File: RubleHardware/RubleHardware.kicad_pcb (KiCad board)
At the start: 4 copper layers, 62 x 46 mm, 49 parts, among them IC1 LTC3780EUH#PBF, J1_IN1 Conn_01x08_Male, J2_OUT1 Conn_01x08_Male

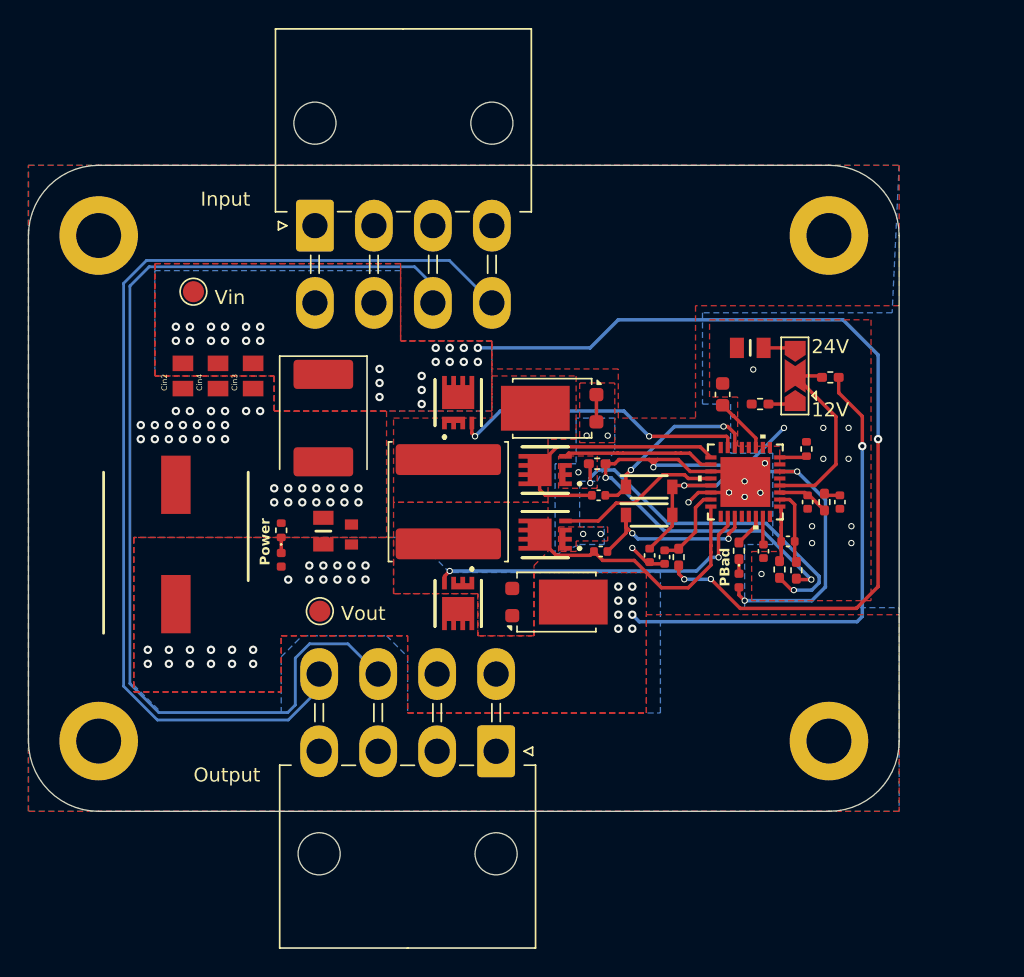
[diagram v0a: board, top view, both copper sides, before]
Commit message: feat: v0.4 ready
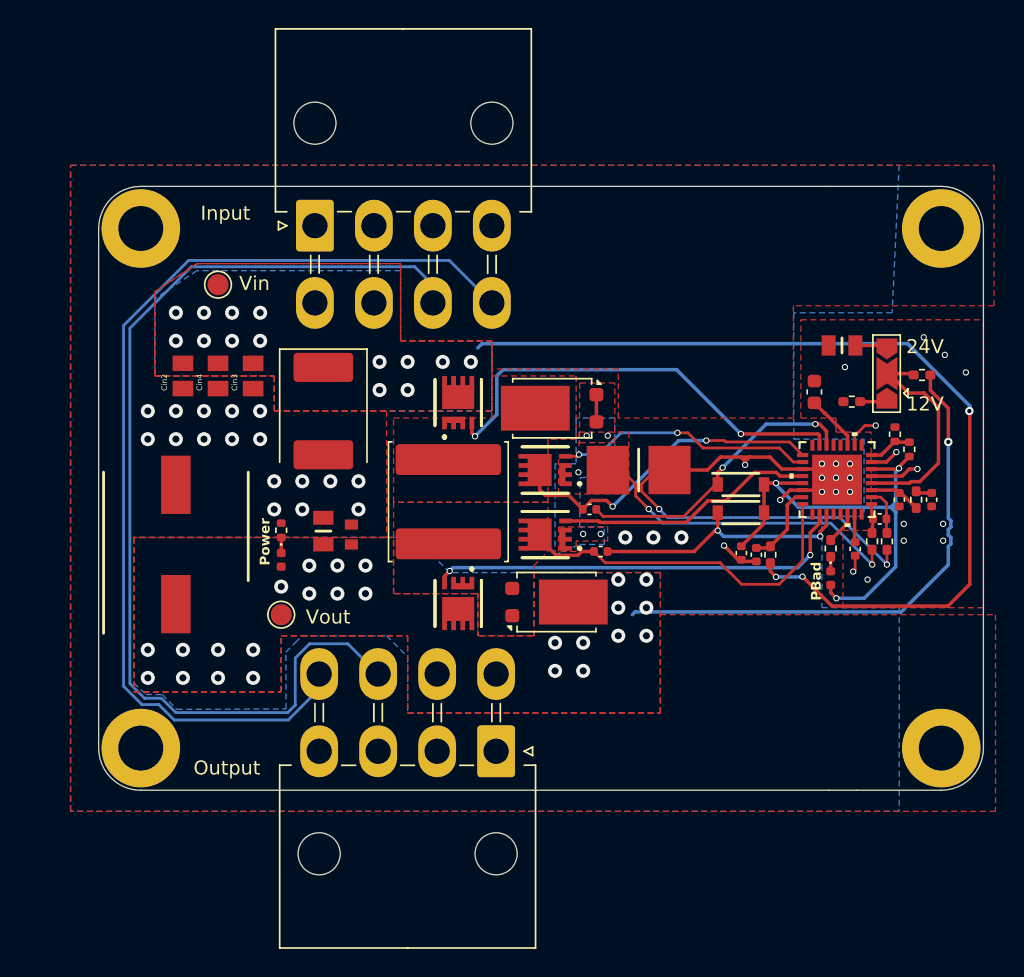
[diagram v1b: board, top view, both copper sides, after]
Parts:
- added R5: 15k, Resistor_SMD:R_0402_1005Metric, F.Cu at (190.7, 83.2)
- Rsense1: value 1.9m -> 5m; footprint Resistor_SMD:R_0402_1005Metric_Pad0.72x0.64mm_HandSolder -> iclr:RESC6432X67N
- moved H3 8.02 mm to (193.0, 67.5)
- moved H4 8.02 mm to (193.0, 104.5)
- moved RSENS+1 6.89 mm to (188.1, 89.8)
- moved RSENS-1 6.77 mm to (189.1, 89.8)
- moved CSENS1 6.72 mm to (188.6, 88.2)
- moved C1 6.53 mm to (192.3, 86.8)
- moved C2 6.53 mm to (190.0, 86.8)
- moved C4 6.53 mm to (184.0, 79.1)
- moved Cf1 6.53 mm to (179.8, 90.7)
- moved Css1 6.53 mm to (186.9, 90.3)
- moved Cvcc1 6.53 mm to (178.8, 90.6)
- moved Da1 6.53 mm to (178.7, 87.7)
- moved Db1 6.53 mm to (178.7, 85.7)
- moved IC1 6.53 mm to (185.6, 85.4)
- moved JP1 6.53 mm to (189.1, 77.8)
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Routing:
- net /TG2: track 21.3 -> 31.8 mm
- net Net-(Db1-K): track 13.0 -> 21.0 mm
- net /BG2: track 10.8 -> 18.4 mm, vias 0 -> 2
- net /BG1: track 11.8 -> 18.5 mm
- net /TG1: track 23.8 -> 30.4 mm
- net /SW1: track 19.0 -> 25.3 mm
- net Net-(Da1-K): track 13.4 -> 19.0 mm
- net /SW2: track 18.7 -> 23.9 mm, vias 0 -> 2
- net GND: track 49.7 -> 54.5 mm, vias 55 -> 47
- net /ICVOUT: track 34.5 -> 38.3 mm, vias 32 -> 26
- net /ICVIN: track 63.4 -> 66.2 mm, vias 29 -> 17
- net /SENS+: track 27.3 -> 25.1 mm
- net Net-(IC1-SENSE-): track 5.34 -> 3.39 mm
- net Net-(IC1-VOSENSE): track 14.1 -> 15.9 mm
- net Net-(IC1-SENSE+): track 3.98 -> 2.11 mm
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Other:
- board size 62 x 46 mm -> 63 x 43 mm
